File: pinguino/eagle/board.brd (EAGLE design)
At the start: 100 x 50.8 mm, 21 parts, among them U1 PIC18F2550-I/SP, U2 LM7805, X1 22MHZ

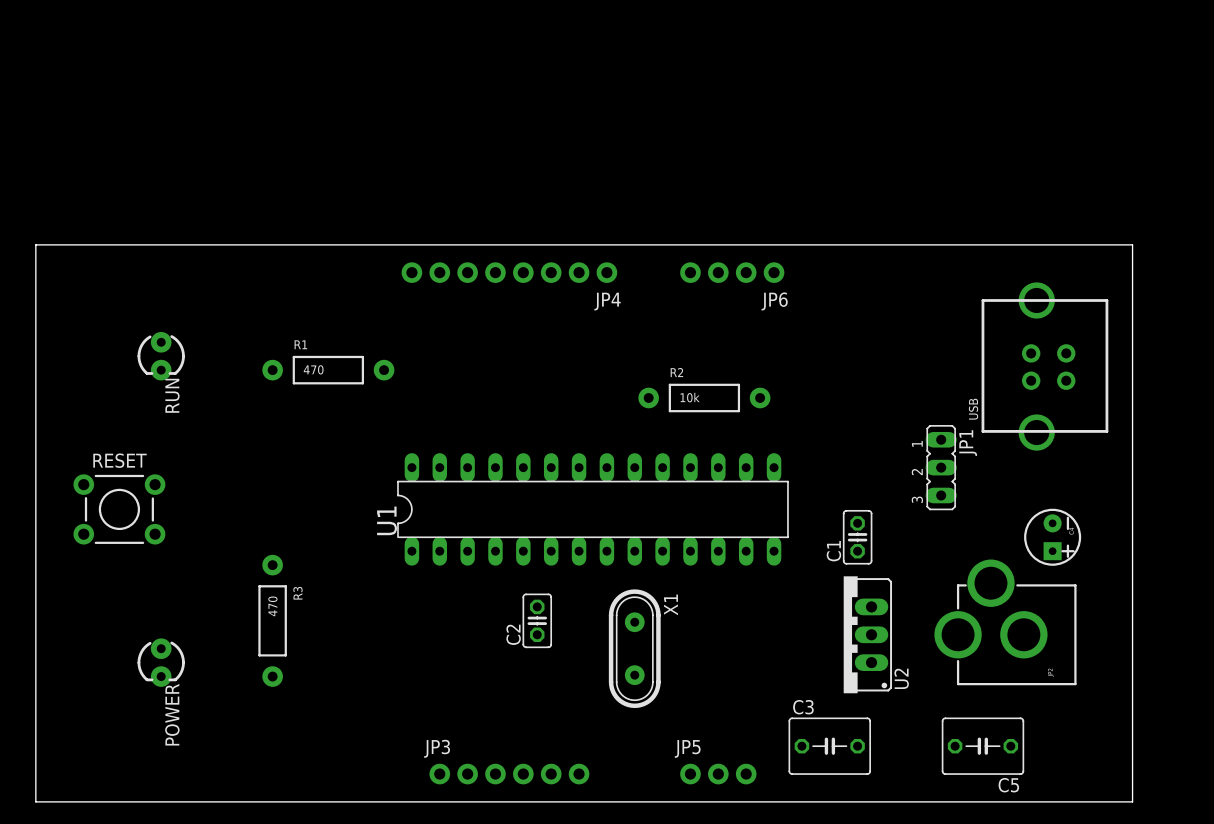
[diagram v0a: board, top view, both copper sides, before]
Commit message: pinguino board
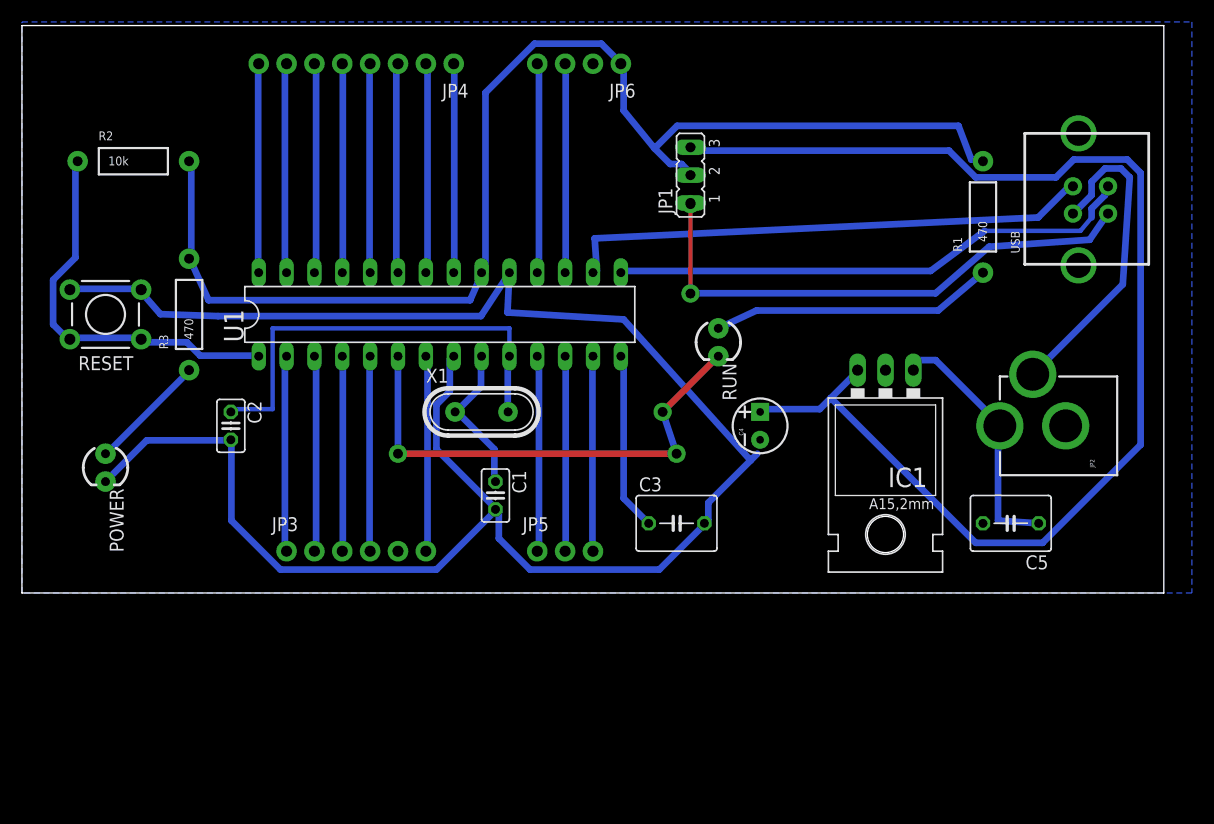
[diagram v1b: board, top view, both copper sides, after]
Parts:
- removed U2: LM7805, v-reg-3:TO220S
- added IC1: (no value), v-reg:78XXL
- moved R1 61.3 mm to (87.6, 82.5), turned to 90 degrees
- moved R2 56.4 mm to (10.2, 87.6)
- moved RUN 50.8 mm to (63.5, 71.1)
- moved JP1 35.1 mm to (61.0, 86.4), turned to 90 degrees
- moved C1 33.2 mm to (43.2, 57.1), turned to 270 degrees
- moved C2 33.1 mm to (19.1, 63.5), turned to 270 degrees
- moved R3 29.0 mm to (15.2, 73.7), turned to 90 degrees
- moved C4 28.5 mm to (67.3, 63.5), turned to 90 degrees
- moved X1 25.7 mm to (41.9, 64.8), turned to 0 degrees
- moved JP3 24.7 mm to (24.1, 52.1)
- moved C3 24.7 mm to (59.7, 54.6)
- moved JP5 24.7 mm to (47.0, 52.1)
- moved JP4 23.6 mm to (39.4, 96.5)
- moved JP6 23.6 mm to (54.6, 96.5)
- moved U1 22.6 mm to (38.1, 73.7)
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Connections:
- removed net N$9: JP3.4
- net GND: now also IC1.GND; no longer U2.1
- net N$10: now also IC1.IN; no longer U2.3
- net N$7: now also IC1.OUT; no longer U2.2
- net PIN5: now also JP3.4
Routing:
- net GND: track 0.00 -> 202.5 mm
- net VCC: track 0.00 -> 117.7 mm
- net N$7: track 0.00 -> 116.3 mm
- net N$8: track 0.00 -> 49.8 mm, vias 0 -> 2
- net D-: track 0.00 -> 48.4 mm
- net D+: track 0.00 -> 48.2 mm
- net PIN6: track 0.00 -> 45.5 mm, vias 0 -> 2
- net N$1: track 0.00 -> 40.8 mm
- net N$4: track 0.00 -> 35.9 mm
- net N$3: track 0.00 -> 25.8 mm
- net N$10: track 0.00 -> 23.8 mm
- net PIN27: track 0.00 -> 19.2 mm
- net PIN23: track 0.00 -> 19.2 mm
- net PIN22: track 0.00 -> 19.2 mm
- net PIN18: track 0.00 -> 19.2 mm
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- added copper zone on layer 16, net GND
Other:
- board size 100 x 50.8 mm -> 104.1 x 51.7 mm
